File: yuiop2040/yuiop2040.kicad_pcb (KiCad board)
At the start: 2 copper layers, 28 x 51 mm, 36 parts, among them J1 USB_B_Micro, J2 USB_C_Receptacle_USB2.0, J3 Conn_01x20, J4 Conn_01x20, J5 Conn_01x03, U1 MIC5219-3.3YM5, U2 RP2040, U3 W25Q16JVSS, Y1 FA238V 12.000000MHz 10.0 +50.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

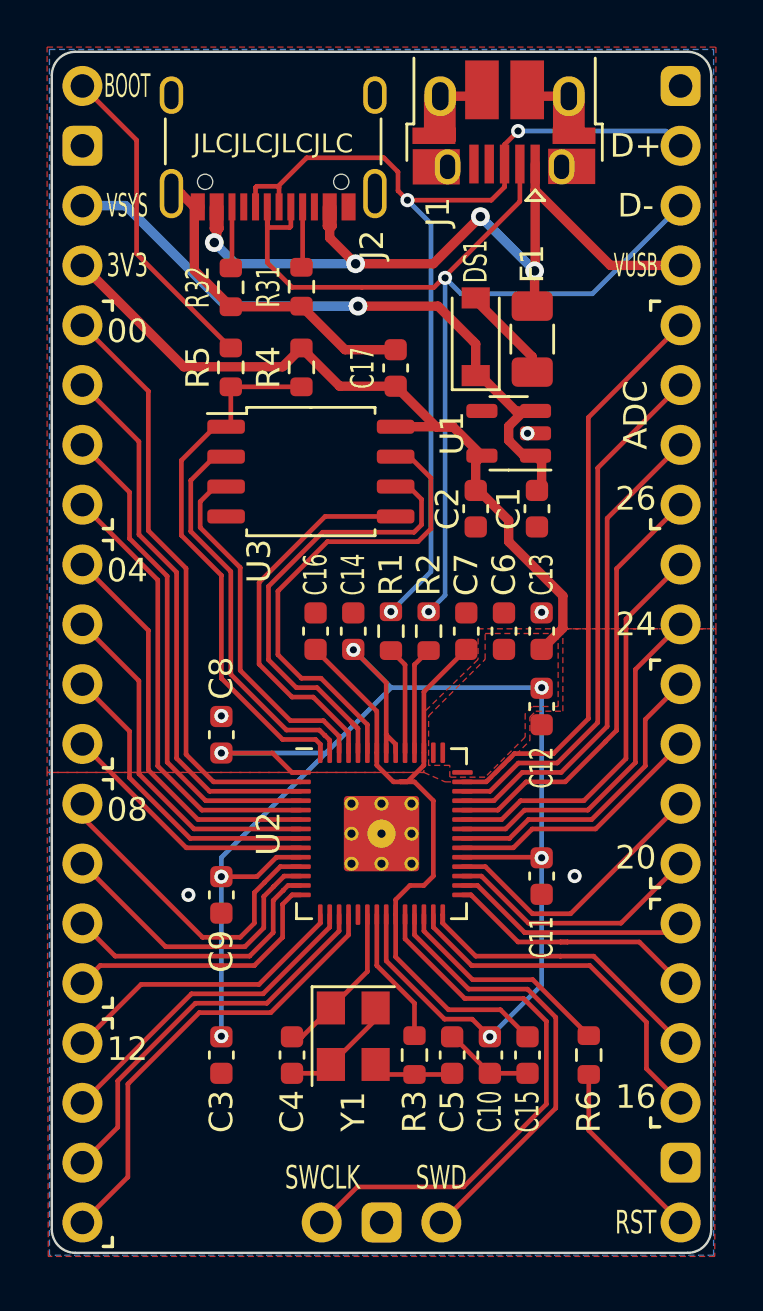
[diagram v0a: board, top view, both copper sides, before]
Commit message: yuiop2040: rev.2
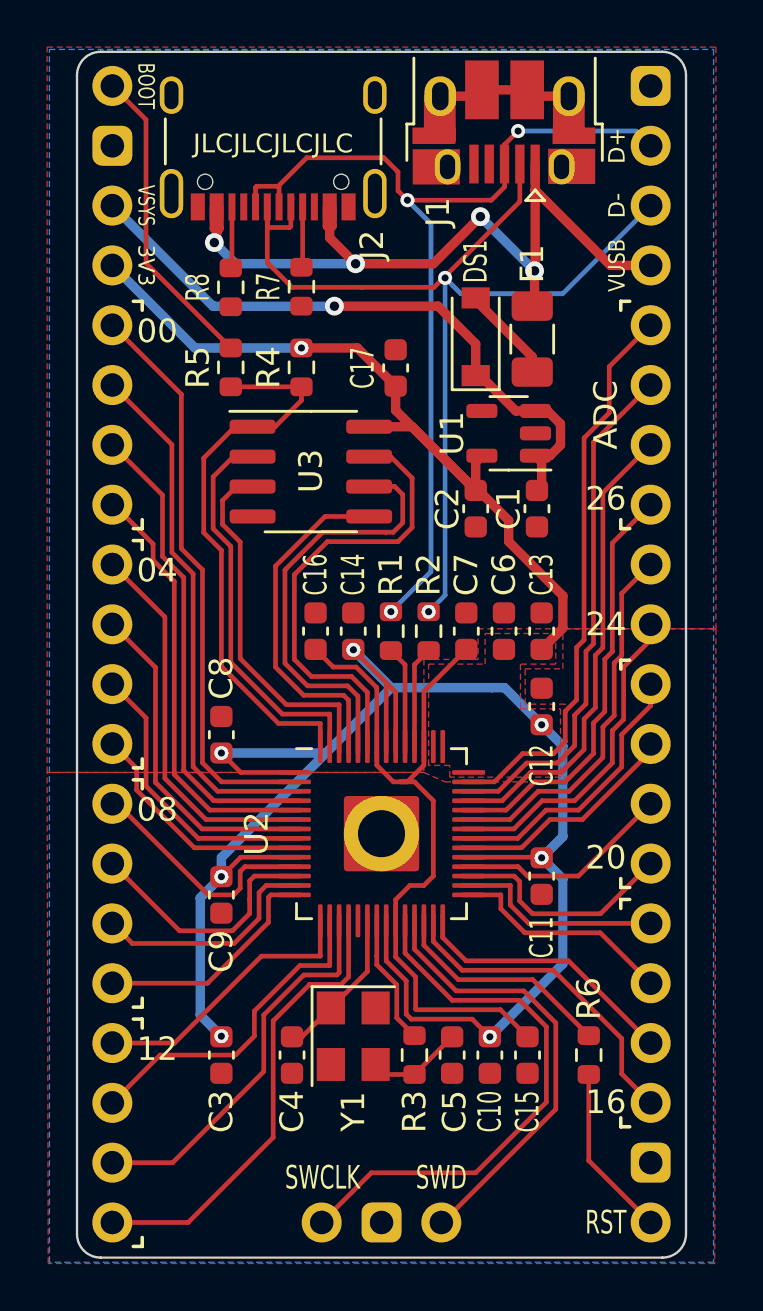
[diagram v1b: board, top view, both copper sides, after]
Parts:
- U2: footprint RP2040_minimal:RP2040-QFN-56 -> RP2040_minimal:RP2040-QFN-56-r2
- U3: footprint Package_SO:SOIC-8_5.23x5.23mm_P1.27mm -> Package_SO:SOIC-8_3.9x4.9mm_P1.27mm
- moved J3 1.27 mm to (128.0, 75.0)
- moved J4 1.27 mm to (150.8, 123.3)
- turned C12 to 90 degrees
- turned C5 to 90 degrees
- renumbered R31 to R7, R32 to R8
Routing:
- net GND: track 26.7 -> 6.18 mm, vias 5 -> 0
- net +3V3: track 105.0 -> 111.7 mm, vias 7 -> 8
- net /GPIO8: track 13.9 -> 10.5 mm
- net /GPIO21: track 12.0 -> 9.43 mm
- net /GPIO10: track 11.9 -> 10.0 mm
- net /GPIO9: track 12.7 -> 11.0 mm
- net /GPIO11: track 11.6 -> 10.2 mm
- net /QSPI_SS: track 22.9 -> 24.3 mm
- net +1V1: track 30.6 -> 32.0 mm
- net /USB_D-: track 45.8 -> 44.5 mm
- net /USB_VBUS: track 35.9 -> 34.6 mm
- net /USB_D+: track 42.6 -> 41.4 mm
- net /VSYS: track 28.6 -> 27.4 mm
- net /QSPI_SD0: track 16.3 -> 15.1 mm
- net /GPIO18: track 11.1 -> 9.89 mm
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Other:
- board size 28 x 51 mm -> 25.9 x 51.2 mm
- board text added: "revision 2"
- board text removed: "designed by KoRoN/KaoriYa"
